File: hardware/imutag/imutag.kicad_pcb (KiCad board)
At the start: 2 copper layers, 18 x 9 mm, 26 parts, among them J201 CONN_02X04, J301 Conn_01x01, J302 Conn_01x01, J303 Conn_01x01, J304 Conn_01x01, J401 CONN_01X02, Q501 Q_NPN_BEC, U1 at25ex321D-UUN, U2 AK09940A, U3 LPS22DF, U302 stm32l431kc, U4 TPS7A2018PDQN, U5 LSM6DSV, U501 RV-3028-C7

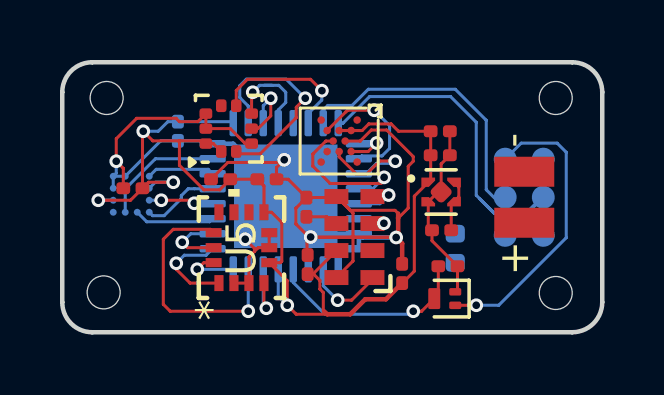
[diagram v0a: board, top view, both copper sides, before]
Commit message: checkpoint
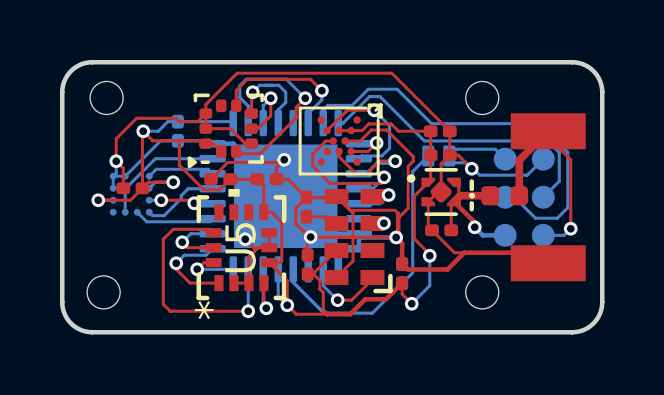
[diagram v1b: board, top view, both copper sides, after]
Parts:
- C502, Q501: moved to B.Cu
- D401: moved to F.Cu
- J401: footprint AccelTag:MS621 -> AccelTag:batterypads
- moved Q501 4.76 mm to (152.6, 107.1)
- moved J301 2.45 mm to (154.0, 111.7)
- moved J302 2.45 mm to (154.0, 105.2)
- moved D401 2.41 mm to (154.8, 108.5), turned to 0 degrees
- moved C502 1.55 mm to (151.3, 111.0), turned to 90 degrees
- moved J401 0.80 mm to (156.2, 108.5), turned to -90 degrees
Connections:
- C7 pad 1: VBAT -> VIN
- D401 pad 1: VBAT -> VIN
- D401 pad 2: VIN -> VBAT
- U4 pad 3: VBAT -> VIN
- U4 pad 4: VBAT -> VIN
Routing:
- net GND: track 57.7 -> 77.0 mm, vias 5 -> 6
- net RST: track 9.86 -> 2.00 mm, vias 1 -> 0
- net VBAT: track 1.81 -> 7.16 mm, vias 0 -> 1
- net VIN: track 0.13 -> 5.46 mm, vias 0 -> 1
- net SWDIO: track 9.49 -> 14.1 mm
- net Net-(Q501-C): track 6.93 -> 11.0 mm, vias 1 -> 0
- net SWCLK: track 12.1 -> 10.2 mm
- net +1V8: track 38.9 -> 40.7 mm, vias 4 -> 6
